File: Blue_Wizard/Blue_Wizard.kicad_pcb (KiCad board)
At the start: 2 copper layers, 108 x 95.2 mm, 47 parts, among them J1 Conn_ARM_JTAG_SWD_10, J10 Left Keywell Header, J11 Conn_01x02, J12 10137062-00021LF, J13 Conn_01x01, J14 Conn_01x02, J2 Conn_01x05, J3 Right FN, J4 Right Keywell, J5 Right Thumb Cluster, J6 Right Keywell Header, J7 Left FN, J8 Left Keywell, J9 Left Thumb Cluster, Q1 BSS84, SW1 SW_Push, U1 BMD-300, U2 MIC5504-3.3YM5, U3 MCP73831T-2ACI_OT, U4 CP2104, Y1 SIT1533AI-H4-DCC-32.768E

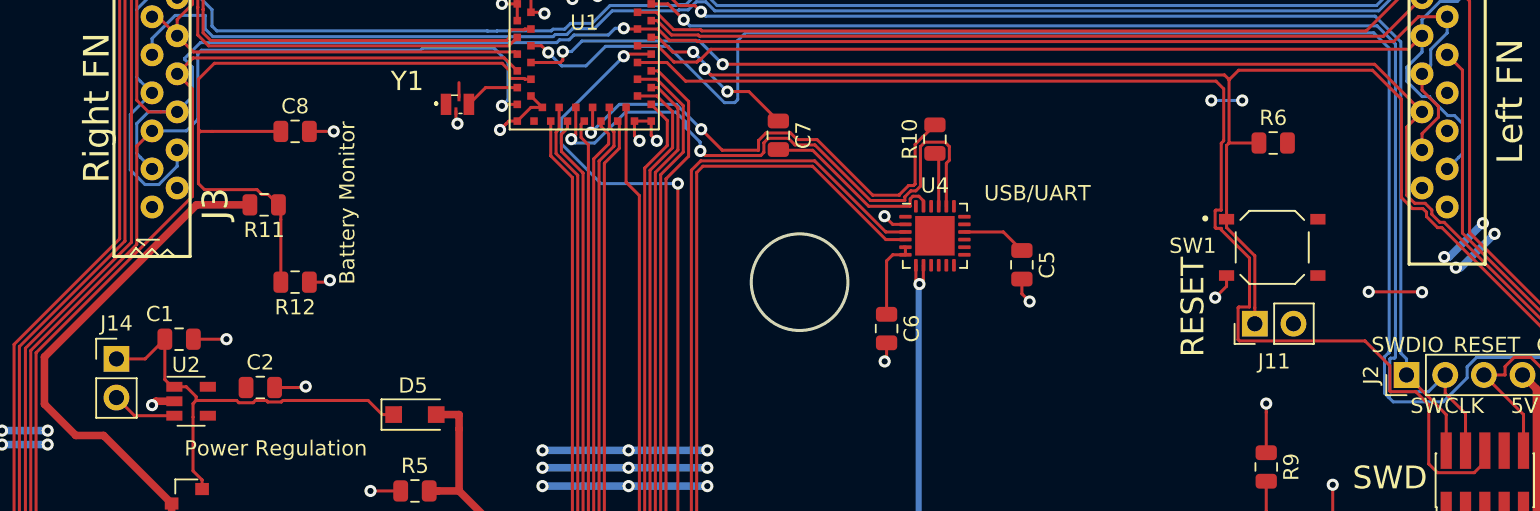
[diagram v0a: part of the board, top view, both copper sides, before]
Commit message: Rev 0a board complete
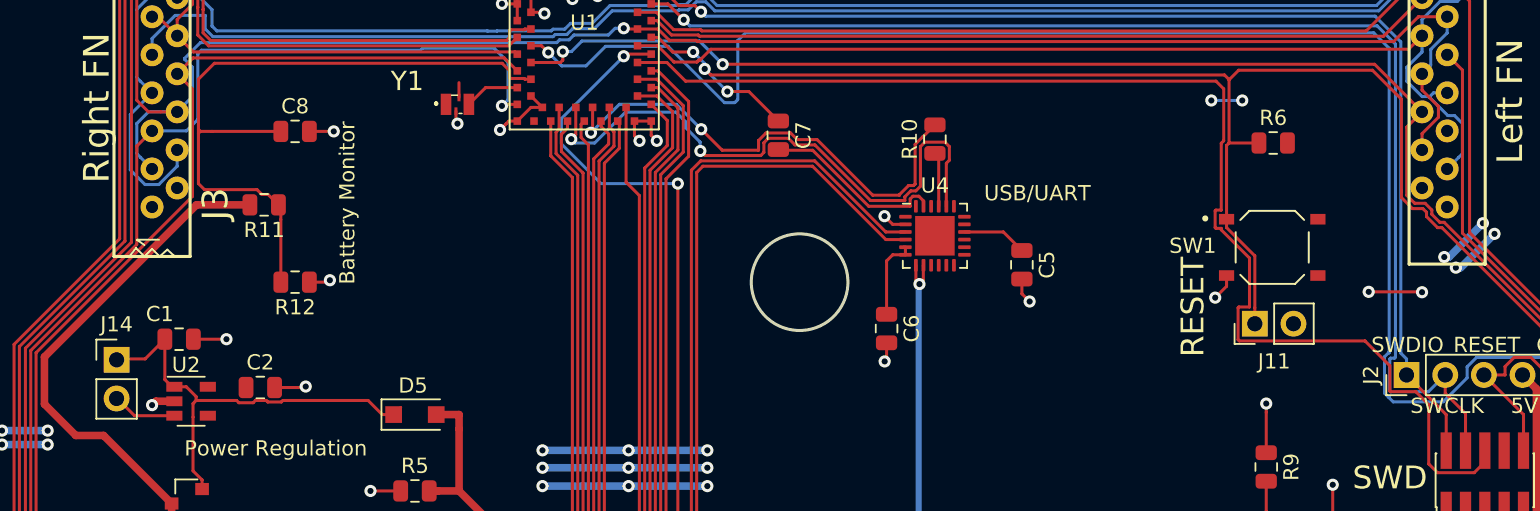
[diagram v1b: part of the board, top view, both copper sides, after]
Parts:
- moved J14 0.06 mm to (105.6, 70.4)
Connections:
- J7 pad 7: Net-(J7-Pad7) -> C6
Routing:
- net C6: track 179.4 -> 180.6 mm
